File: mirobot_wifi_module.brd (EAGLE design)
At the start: 27.9 x 34 mm, 4 parts

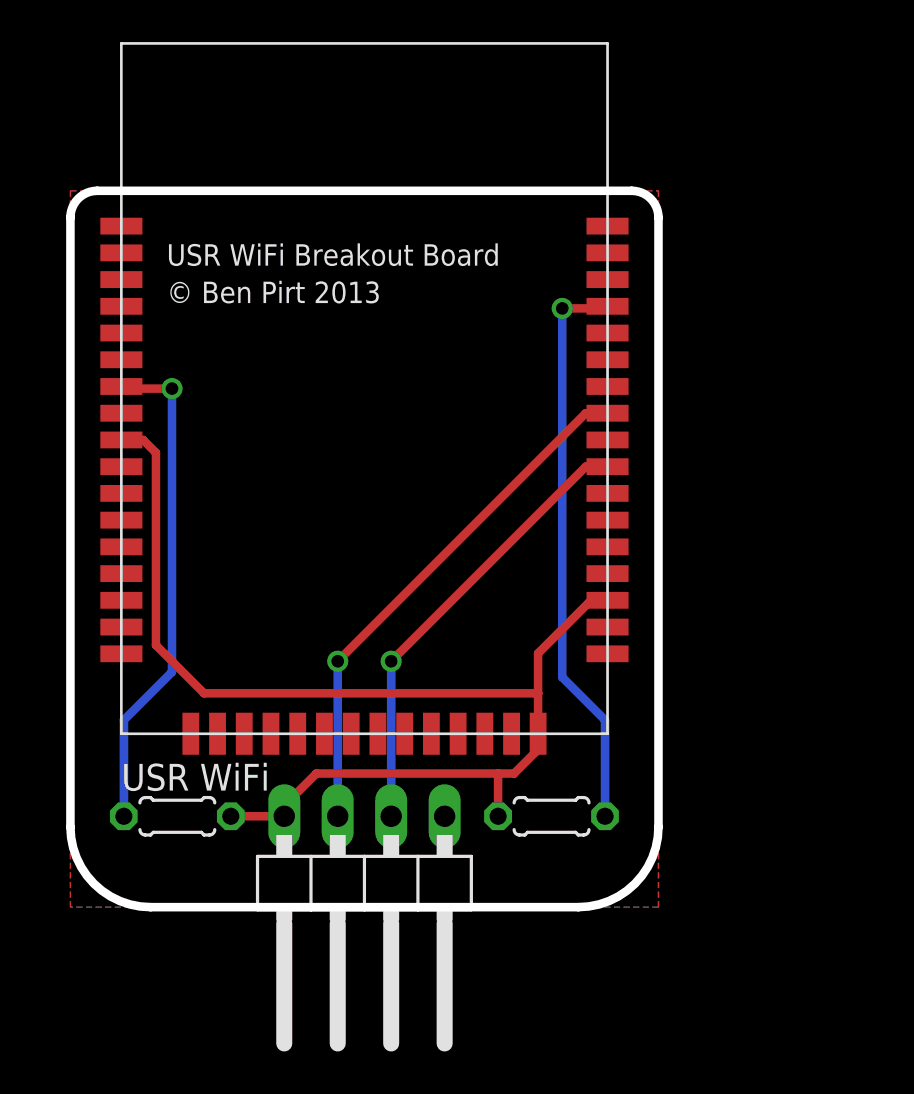
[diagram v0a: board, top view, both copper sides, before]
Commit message: Version 1.4 of the mian PCB and 1.1 of the WiFi PCB
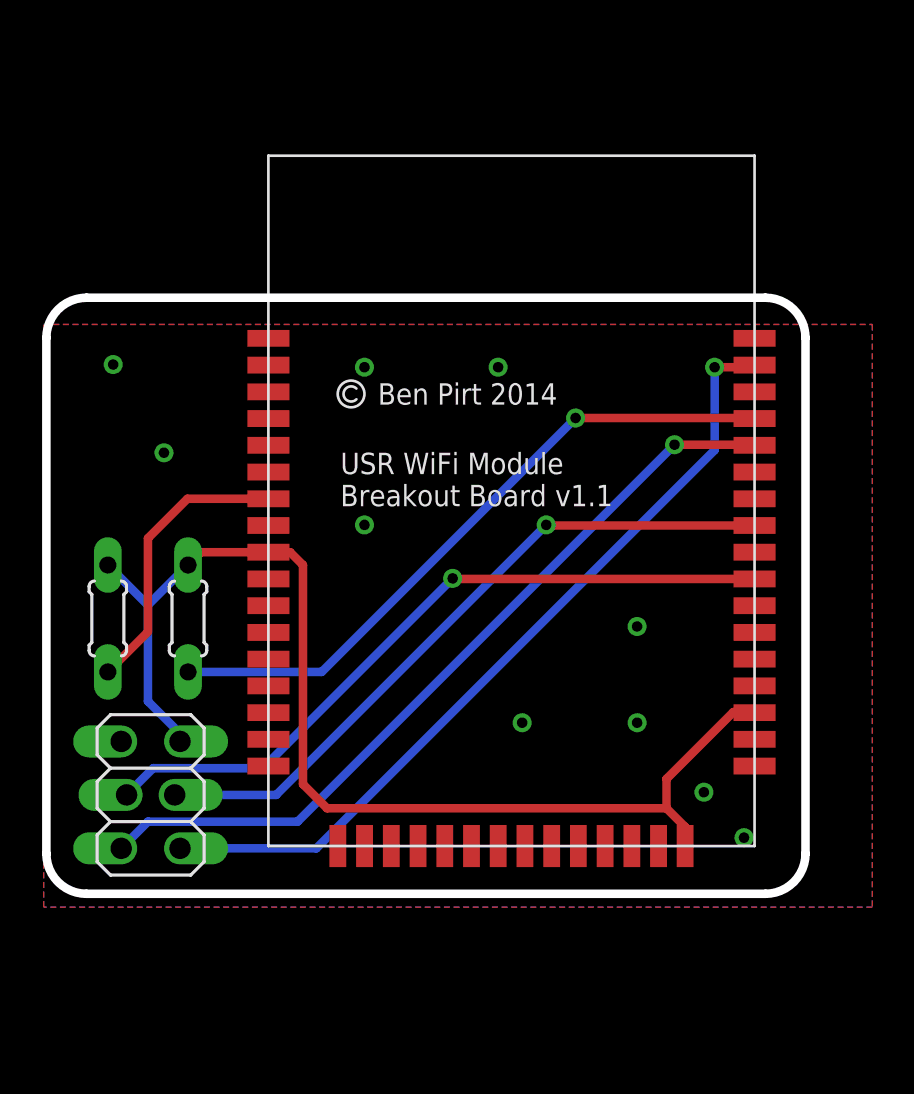
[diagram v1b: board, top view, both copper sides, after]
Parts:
- JP1: device pinhead:1X04/90 -> Child-Friendly-Parts:2X03
- R1, R2: device rcl:0204/5 -> Child-Friendly-Parts:0204/5
- moved R1 19.7 mm to (6.86, 13.2), turned to 90 degrees
- moved JP1 11.2 mm to (5.08, 4.83), turned to 270 degrees
- moved R2 9.96 mm to (3.05, 13.2), turned to 270 degrees
- moved U$1 8.79 mm to (22.2, 18.8)
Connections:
- new net N$6: JP1.5, U$1.NREADY
- new net N$7: JP1.6, U$1.EXT_RESET
- net N$2: now also JP1.2; no longer JP1.4
- net N$3: now also JP1.4; no longer JP1.3
- net N$5: now also JP1.3; no longer JP1.2
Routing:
- net N$7: track 0.00 -> 40.2 mm, vias 0 -> 1
- net N$6: track 0.00 -> 39.3 mm, vias 0 -> 1
- net N$5: track 21.5 -> 34.3 mm
- net N$1: track 23.7 -> 13.6 mm, vias 1 -> 0
- net N$3: track 25.1 -> 32.9 mm
- net N$4: track 27.2 -> 33.1 mm
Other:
- board size 27.9 x 34 mm -> 36.1 x 28.3 mm
- board text added: "Ben Pirt 2014"
- board text added: "USR WiFi Module Breakout Board v1.1"
- board text removed: "USR WiFi Breakout Board"
- board text removed: "© Ben Pirt 2013"
